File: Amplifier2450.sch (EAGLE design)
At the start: 17 parts, among them X1 SMA-142-0701-801/806, X2 SMA-142-0701-801/806

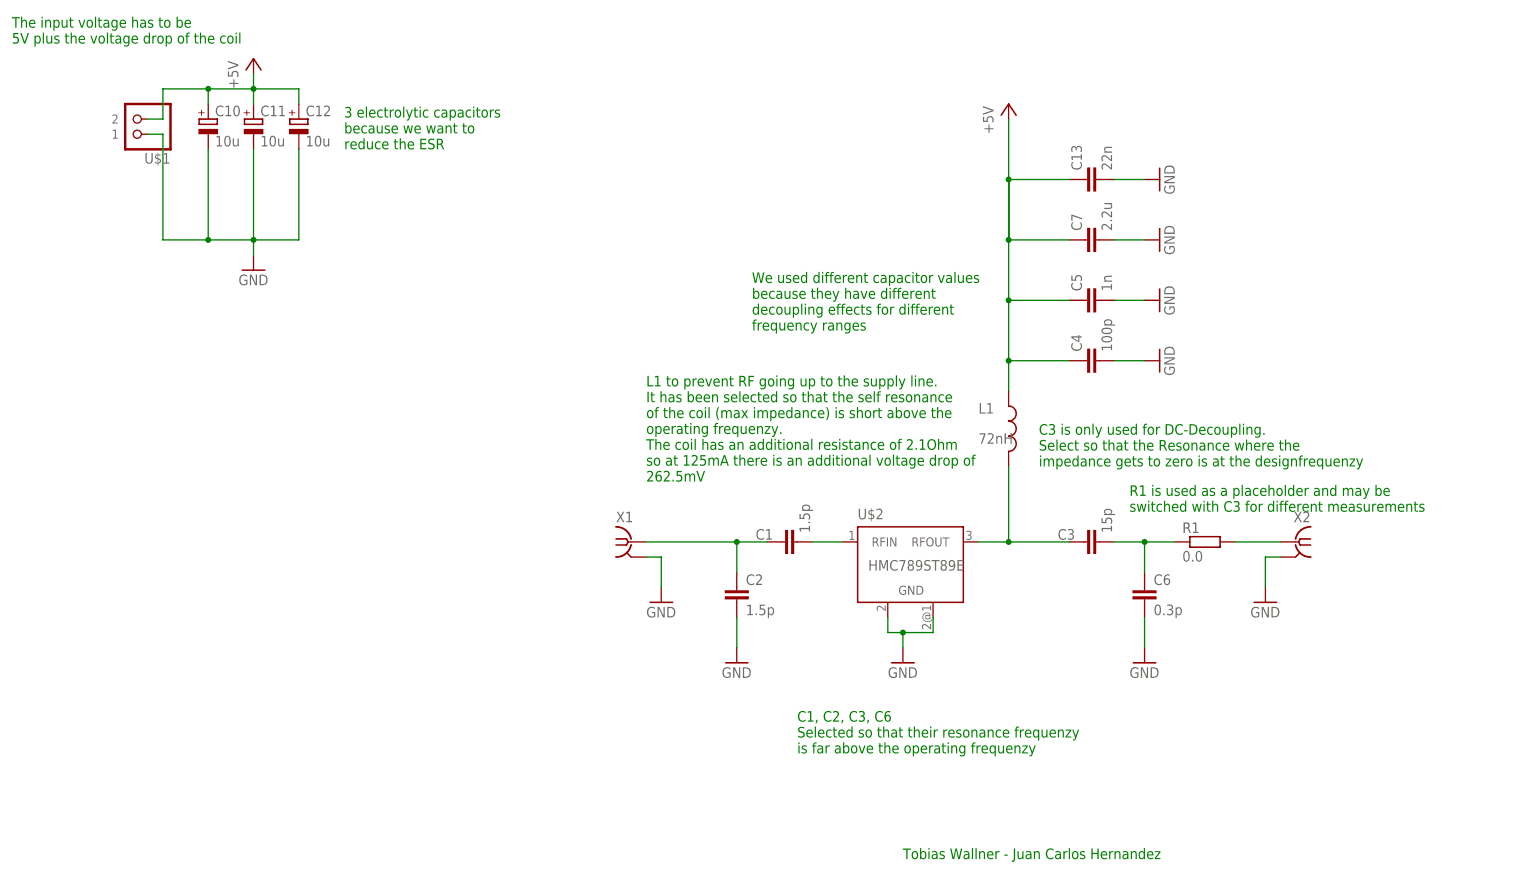
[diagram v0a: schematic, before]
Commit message: (Tobias): made finishing touches to the design
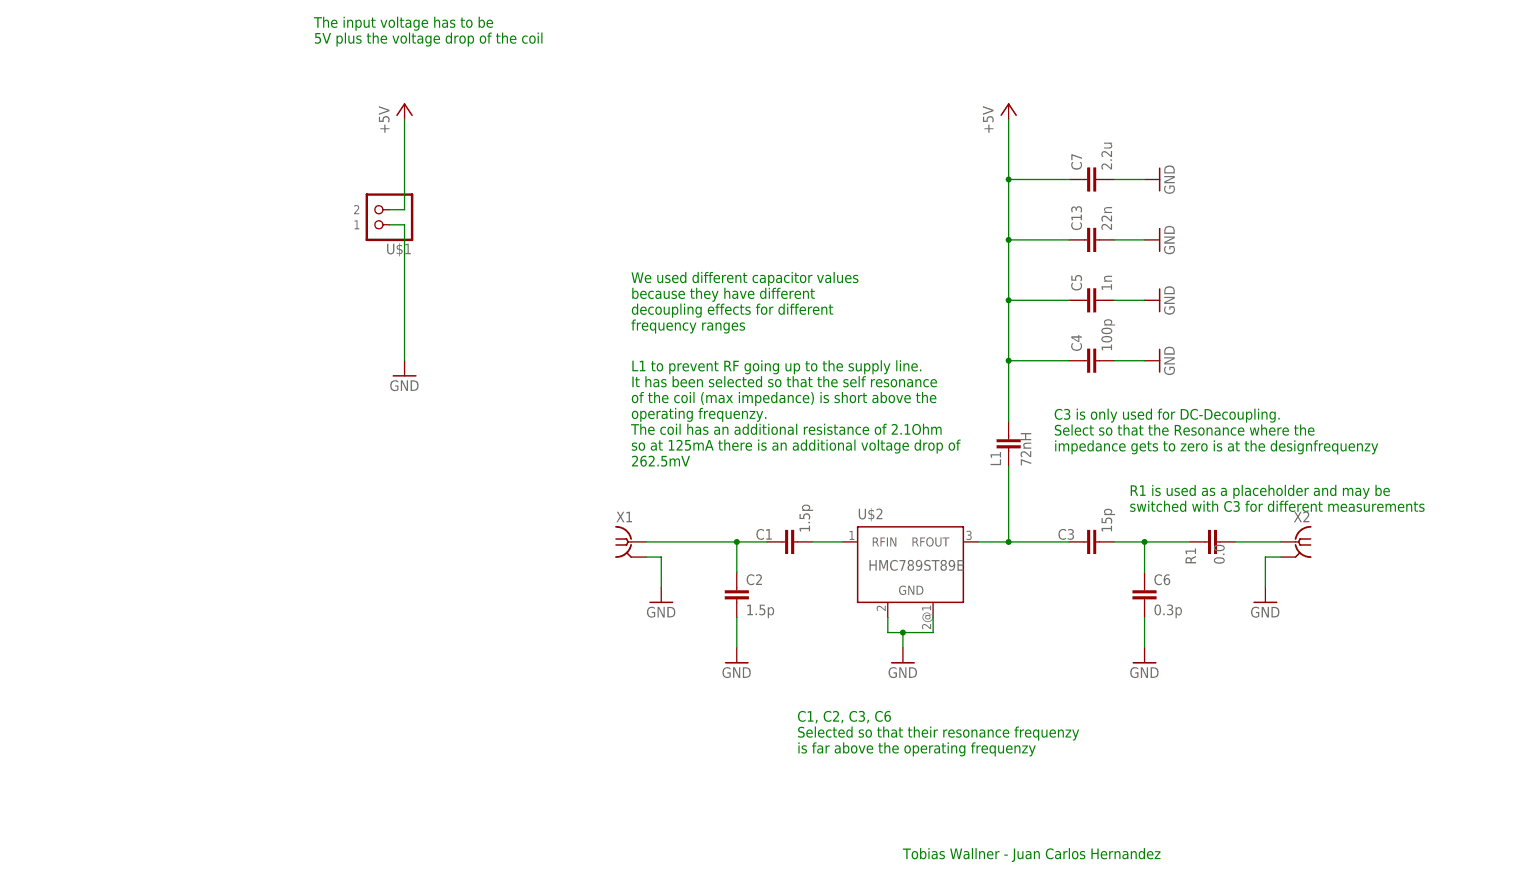
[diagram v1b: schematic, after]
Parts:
- removed C10, C11, C12: 10u, rcl:CPOL-EUE2.5-5
- C1, C2, C3, C6: device rcl:C-EUC0402 -> rcl:C-EUC0603
- L1: device own_htl3r-discrete-1:L_US_ -> rcl:C-EUC0603
- R1: device rcl:R-EU_R0402 -> rcl:C-EUC0603
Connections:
- net +5V: no longer C10.+, C11.+, C12.+
- net GND: no longer C10.-, C11.-, C12.-
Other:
- note removed: "3 electrolytic capacitors because we want to reduce the ESR"
- moved on the sheet: C13, C7, R1, U$1
